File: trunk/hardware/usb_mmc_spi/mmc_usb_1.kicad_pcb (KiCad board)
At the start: 2 copper layers, 47.6 x 27.3 mm, 25 parts, among them J301 MINI-USB-5P-3400020P1, K301 CONN_3, P301 CONN_5X2, P302 MICRO-SDCARD-CONNECTOR-330006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, P303 CONN_10X2, P304 CONN_10X2, P305 CONN_1, P306 CONN_1, U301 FT232RL

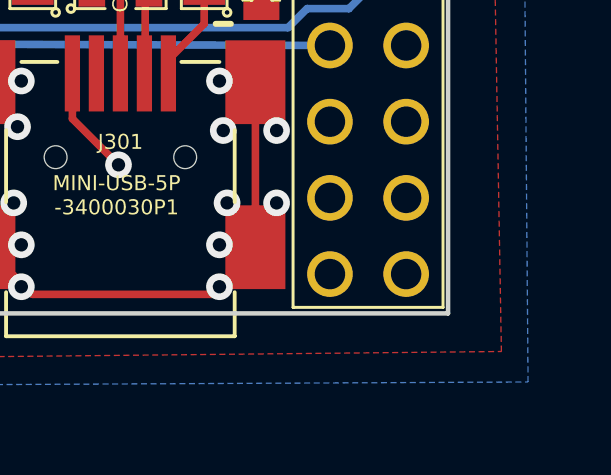
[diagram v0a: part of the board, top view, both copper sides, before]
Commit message: bugfix
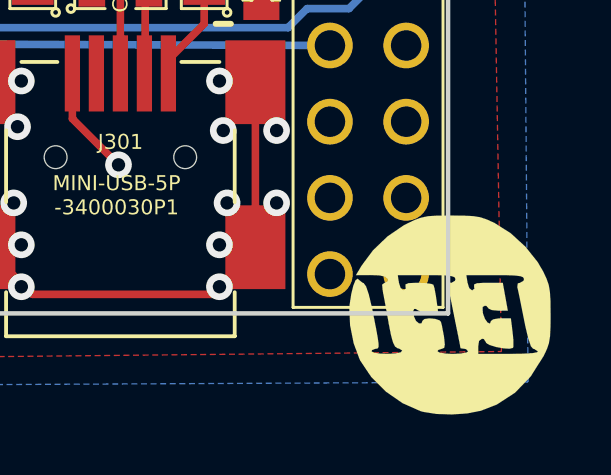
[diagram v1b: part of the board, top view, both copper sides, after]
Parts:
- added G301: LOGO, LOGO_F, F.Cu at (224.1, 179.2)
- renumbered G301 to G3
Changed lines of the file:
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@@
     (links 76)
     (no_connects 0)
-    (area 120.549999 93.244999 233.0704 190.600001)
+    (area 176.327999 151.689999 224.103001 179.145001)
     (thickness 1.6)
     (drawings 62)
     (tracks 536)
     (zones 0)
-    (modules 25)
+    (modules 26)
     (nets 24)
   )
@@
       (layers F.Cu F.Paste F.Mask)
     )
-    (pad G301 smd rect (at -6.893 8.032 270) (size 1.524 1.016)
+    (pad G3 smd rect (at -6.893 8.032 270) (size 1.524 1.016)
       (layers F.Cu F.Paste F.Mask)
       (net 13 GND)
@@
   (module LOGO_F (layer B.Cu)
     (at 201.549 165.608)
-    (fp_text reference G301 (at 0 -4.14782) (layer B.SilkS) hide
+    (fp_text reference G3 (at 0 -4.14782) (layer B.SilkS) hide
       (effects (font (size 1.524 1.524) (thickness 0.3048)) (justify mirror))
     )
@@
     )
   )
+  (module LOGO_F (layer F.Cu)
+    (at 224.103001 179.150001)
+    (fp_text reference G301 (at 0 4.14782) (layer F.SilkS) hide
+      (effects (font (size 1.524 1.524) (thickness 0.3048)))
+    )
+    (fp_text value LOGO (at 0 -4.14782) (layer F.SilkS) hide
+      (effects (font (size 1.524 1.524) (thickness 0.3048)))
+    )
+    (fp_poly (pts (xy 3.34518 -0.04318) (xy 3.3401 0.381) (xy 3.32486 0.68326) (xy 3.28676 0.90932)
+      (xy 3.22326 1.1049) (xy 3.12166 1.3208) (xy 3.10896 1.3462) (xy 2.921 1.64084)
+      (xy 2.921 1.18618) (xy 2.79654 1.1049) (xy 2.75844 1.09982) (xy 2.68732 1.016)
+      (xy 2.60096 0.76708) (xy 2.5019 0.35052) (xy 2.46126 0.14732) (xy 2.38252 -0.24638)
+      (xy 2.31394 -0.58928) (xy 2.2606 -0.84074) (xy 2.23266 -0.9525) (xy 2.2479 -1.07696)
+      (xy 2.32156 -1.09982) (xy 2.4384 -1.16586) (xy 2.45618 -1.22682) (xy 2.42824 -1.28524)
+      (xy 2.33172 -1.3208) (xy 2.13868 -1.34366) (xy 1.82372 -1.35382) (xy 1.49606 -1.35382)
+      (xy 0.53594 -1.35382) (xy 0.57404 -1.09982) (xy 0.63246 -0.92202) (xy 0.7239 -0.84836)
+      (xy 0.72644 -0.84582) (xy 0.80264 -0.90678) (xy 0.79248 -0.97536) (xy 0.79248 -1.04648)
+      (xy 0.889 -1.08458) (xy 1.10744 -1.09982) (xy 1.24714 -1.09982) (xy 1.75006 -1.09982)
+      (xy 1.83388 -0.635) (xy 1.9177 -0.17018) (xy 1.59258 -0.17018) (xy 1.38684 -0.1905)
+      (xy 1.27508 -0.23876) (xy 1.27 -0.254) (xy 1.20142 -0.3302) (xy 1.15316 -0.33782)
+      (xy 1.0795 -0.2921) (xy 1.08204 -0.127) (xy 1.0922 -0.07112) (xy 1.1557 0.1016)
+      (xy 1.24206 0.22352) (xy 1.3208 0.25908) (xy 1.35382 0.1778) (xy 1.35382 0.17526)
+      (xy 1.43002 0.11684) (xy 1.61544 0.08636) (xy 1.68656 0.08382) (xy 2.0193 0.08382)
+      (xy 2.07772 0.55372) (xy 2.10312 0.81788) (xy 2.10312 1.01092) (xy 2.09042 1.06934)
+      (xy 1.9685 1.09982) (xy 1.76022 1.08458) (xy 1.52146 1.03886) (xy 1.31318 0.97536)
+      (xy 1.1938 0.90424) (xy 1.18618 0.88138) (xy 1.1176 0.7747) (xy 1.05918 0.762)
+      (xy 0.95758 0.8382) (xy 0.93218 1.016) (xy 0.93218 1.27) (xy 1.95072 1.27)
+      (xy 2.42062 1.26238) (xy 2.74066 1.2446) (xy 2.90322 1.21158) (xy 2.921 1.18618)
+      (xy 2.921 1.64084) (xy 2.67716 2.02692) (xy 2.15646 2.5654) (xy 1.5494 2.9591)
+      (xy 1.02108 3.16484) (xy 0.59182 3.24866) (xy 0.59182 1.18618) (xy 0.52324 1.10998)
+      (xy 0.46482 1.09982) (xy 0.35306 1.08458) (xy 0.33782 1.06934) (xy 0.32258 0.98044)
+      (xy 0.2794 0.75692) (xy 0.21336 0.4318) (xy 0.13462 0.04064) (xy 0.127 0)
+      (xy 0.03556 -0.44958) (xy -0.02794 -0.75692) (xy -0.06096 -0.94996) (xy -0.06858 -1.0541)
+      (xy -0.05334 -1.09728) (xy -0.01524 -1.1049) (xy 0.04318 -1.09982) (xy 0.15494 -1.1684)
+      (xy 0.17018 -1.22682) (xy 0.14224 -1.28524) (xy 0.04572 -1.3208) (xy -0.14732 -1.34366)
+      (xy -0.46228 -1.35382) (xy -0.78994 -1.35382) (xy -1.75006 -1.35382) (xy -1.71196 -1.09982)
+      (xy -1.65354 -0.92202) (xy -1.5621 -0.84836) (xy -1.55956 -0.84582) (xy -1.48336 -0.90678)
+      (xy -1.49352 -0.97282) (xy -1.49098 -1.04902) (xy -1.39446 -1.08712) (xy -1.1684 -1.09982)
+      (xy -1.07188 -1.09982) (xy -0.80772 -1.08966) (xy -0.61976 -1.05918) (xy -0.56134 -1.03378)
+      (xy -0.52578 -0.9144) (xy -0.48514 -0.69088) (xy -0.45974 -0.52578) (xy -0.40132 -0.08382)
+      (xy -0.69342 -0.08382) (xy -0.91948 -0.11176) (xy -1.07696 -0.18034) (xy -1.08204 -0.18542)
+      (xy -1.1938 -0.254) (xy -1.2319 -0.17018) (xy -1.21158 0.02032) (xy -1.143 0.17018)
+      (xy -1.04394 0.254) (xy -0.95758 0.24892) (xy -0.93218 0.17018) (xy -0.86106 0.10668)
+      (xy -0.69596 0.08382) (xy -0.50546 0.1016) (xy -0.35306 0.15494) (xy -0.31242 0.20066)
+      (xy -0.27432 0.35052) (xy -0.2286 0.59436) (xy -0.20828 0.70866) (xy -0.18288 0.94996)
+      (xy -0.20066 1.0668) (xy -0.27686 1.09982) (xy -0.28702 1.09982) (xy -0.4064 1.143)
+      (xy -0.42418 1.18618) (xy -0.34544 1.22936) (xy -0.14478 1.25984) (xy 0.08382 1.27)
+      (xy 0.3556 1.2573) (xy 0.53848 1.22428) (xy 0.59182 1.18618) (xy 0.59182 3.24866)
+      (xy 0.5715 3.25374) (xy 0.0508 3.2893) (xy -0.4699 3.27152) (xy -0.91694 3.2004)
+      (xy -0.99314 3.17754) (xy -1.59004 2.91338) (xy -2.15392 2.52222) (xy -2.63652 2.03708)
+      (xy -2.99974 1.49606) (xy -3.03022 1.43256) (xy -3.22326 0.90932) (xy -3.3401 0.32258)
+      (xy -3.3655 -0.2413) (xy -3.3528 -0.39624) (xy -3.29946 -0.7366) (xy -3.23088 -1.01092)
+      (xy -3.15722 -1.18872) (xy -3.0861 -1.23698) (xy -3.06578 -1.21666) (xy -2.93624 -1.10998)
+      (xy -2.88544 -1.08712) (xy -2.80924 -0.98298) (xy -2.7178 -0.71374) (xy -2.6162 -0.2921)
+      (xy -2.57302 -0.08128) (xy -2.48158 0.38354) (xy -2.42316 0.70612) (xy -2.39268 0.9144)
+      (xy -2.39014 1.03124) (xy -2.41554 1.08458) (xy -2.4638 1.09982) (xy -2.49682 1.09982)
+      (xy -2.61112 1.14554) (xy -2.62382 1.18618) (xy -2.54762 1.22936) (xy -2.34696 1.25984)
+      (xy -2.11582 1.27) (xy -1.8288 1.25476) (xy -1.651 1.21412) (xy -1.60274 1.15824)
+      (xy -1.7018 1.09728) (xy -1.76276 1.0795) (xy -1.8415 1.02362) (xy -1.91008 0.88646)
+      (xy -1.97866 0.63754) (xy -2.05486 0.25146) (xy -2.06248 0.2032) (xy -2.13106 -0.18288)
+      (xy -2.19456 -0.52578) (xy -2.24282 -0.78232) (xy -2.25806 -0.86868) (xy -2.27076 -1.0414)
+      (xy -2.19202 -1.09982) (xy -2.1717 -1.10236) (xy -2.07772 -1.15316) (xy -2.08534 -1.22936)
+      (xy -2.1717 -1.30556) (xy -2.36728 -1.3462) (xy -2.6416 -1.35636) (xy -3.14706 -1.35382)
+      (xy -2.95656 -1.67132) (xy -2.5781 -2.18186) (xy -2.09296 -2.64668) (xy -1.55702 -3.01244)
+      (xy -1.44018 -3.0734) (xy -1.18618 -3.19532) (xy -0.97536 -3.27152) (xy -0.75692 -3.31724)
+      (xy -0.48514 -3.33756) (xy -0.10668 -3.34264) (xy 0.04064 -3.34264) (xy 0.46482 -3.33756)
+      (xy 0.76962 -3.32232) (xy 1.00076 -3.28422) (xy 1.2065 -3.21564) (xy 1.43764 -3.1115)
+      (xy 1.47574 -3.09372) (xy 2.00914 -2.7559) (xy 2.50444 -2.30378) (xy 2.91592 -1.78816)
+      (xy 3.10134 -1.46812) (xy 3.21056 -1.2319) (xy 3.28168 -1.02616) (xy 3.31978 -0.8001)
+      (xy 3.3401 -0.50546) (xy 3.34264 -0.09398) (xy 3.34518 -0.04318) (xy 3.34518 -0.04318)) (layer F.SilkS) (width 0.00254))
+  )
   (gr_text 6 (at 215.519 158.623) (layer B.SilkS)

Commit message: kinda fixing the whole G* situation
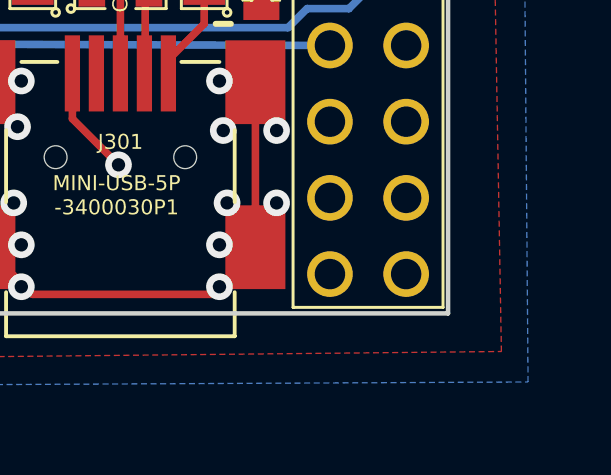
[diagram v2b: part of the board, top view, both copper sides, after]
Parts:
- removed G301: LOGO, LOGO_F
- renumbered G3 to G305
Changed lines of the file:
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@@
     (links 76)
     (no_connects 0)
-    (area 176.327999 151.689999 224.103001 179.145001)
+    (area 120.549999 93.244999 233.0704 190.600001)
     (thickness 1.6)
     (drawings 62)
     (tracks 536)
     (zones 0)
-    (modules 26)
+    (modules 25)
     (nets 24)
   )
@@
       (layers F.Cu F.Paste F.Mask)
     )
-    (pad G3 smd rect (at -6.893 8.032 270) (size 1.524 1.016)
-      (layers F.Cu F.Paste F.Mask)
-      (net 13 GND)
-    )
-    (pad G2 smd rect (at 2.88 7.686 270) (size 2.032 1.524)
-      (layers F.Cu F.Paste F.Mask)
-      (net 13 GND)
-    )
-    (pad G3 smd rect (at 2.88 -7.714 270) (size 2.032 1.524)
-      (layers F.Cu F.Paste F.Mask)
-      (net 13 GND)
-    )
-    (pad G4 smd rect (at -7.101 -6.895 270) (size 1.524 1.524)
+    (pad G301 smd rect (at -6.893 8.032 270) (size 1.524 1.016)
+      (layers F.Cu F.Paste F.Mask)
+      (net 13 GND)
+    )
+    (pad G302 smd rect (at 2.88 7.686 270) (size 2.032 1.524)
+      (layers F.Cu F.Paste F.Mask)
+      (net 13 GND)
+    )
+    (pad G303 smd rect (at 2.88 -7.714 270) (size 2.032 1.524)
+      (layers F.Cu F.Paste F.Mask)
+      (net 13 GND)
+    )
+    (pad G304 smd rect (at -7.101 -6.895 270) (size 1.524 1.524)
       (layers F.Cu F.Paste F.Mask)
       (net 13 GND)
@@
   (module LOGO_F (layer B.Cu)
     (at 201.549 165.608)
-    (fp_text reference G3 (at 0 -4.14782) (layer B.SilkS) hide
+    (fp_text reference G305 (at 0 -4.14782) (layer B.SilkS) hide
       (effects (font (size 1.524 1.524) (thickness 0.3048)) (justify mirror))
     )
@@
     )
   )
-  (module LOGO_F (layer F.Cu)
-    (at 224.103001 179.150001)
-    (fp_text reference G301 (at 0 4.14782) (layer F.SilkS) hide
-      (effects (font (size 1.524 1.524) (thickness 0.3048)))
-    )
-    (fp_text value LOGO (at 0 -4.14782) (layer F.SilkS) hide
-      (effects (font (size 1.524 1.524) (thickness 0.3048)))
-    )
-    (fp_poly (pts (xy 3.34518 -0.04318) (xy 3.3401 0.381) (xy 3.32486 0.68326) (xy 3.28676 0.90932)
-      (xy 3.22326 1.1049) (xy 3.12166 1.3208) (xy 3.10896 1.3462) (xy 2.921 1.64084)
-      (xy 2.921 1.18618) (xy 2.79654 1.1049) (xy 2.75844 1.09982) (xy 2.68732 1.016)
-      (xy 2.60096 0.76708) (xy 2.5019 0.35052) (xy 2.46126 0.14732) (xy 2.38252 -0.24638)
-      (xy 2.31394 -0.58928) (xy 2.2606 -0.84074) (xy 2.23266 -0.9525) (xy 2.2479 -1.07696)
-      (xy 2.32156 -1.09982) (xy 2.4384 -1.16586) (xy 2.45618 -1.22682) (xy 2.42824 -1.28524)
-      (xy 2.33172 -1.3208) (xy 2.13868 -1.34366) (xy 1.82372 -1.35382) (xy 1.49606 -1.35382)
-      (xy 0.53594 -1.35382) (xy 0.57404 -1.09982) (xy 0.63246 -0.92202) (xy 0.7239 -0.84836)
-      (xy 0.72644 -0.84582) (xy 0.80264 -0.90678) (xy 0.79248 -0.97536) (xy 0.79248 -1.04648)
-      (xy 0.889 -1.08458) (xy 1.10744 -1.09982) (xy 1.24714 -1.09982) (xy 1.75006 -1.09982)
-      (xy 1.83388 -0.635) (xy 1.9177 -0.17018) (xy 1.59258 -0.17018) (xy 1.38684 -0.1905)
-      (xy 1.27508 -0.23876) (xy 1.27 -0.254) (xy 1.20142 -0.3302) (xy 1.15316 -0.33782)
-      (xy 1.0795 -0.2921) (xy 1.08204 -0.127) (xy 1.0922 -0.07112) (xy 1.1557 0.1016)
-      (xy 1.24206 0.22352) (xy 1.3208 0.25908) (xy 1.35382 0.1778) (xy 1.35382 0.17526)
-      (xy 1.43002 0.11684) (xy 1.61544 0.08636) (xy 1.68656 0.08382) (xy 2.0193 0.08382)
-      (xy 2.07772 0.55372) (xy 2.10312 0.81788) (xy 2.10312 1.01092) (xy 2.09042 1.06934)
-      (xy 1.9685 1.09982) (xy 1.76022 1.08458) (xy 1.52146 1.03886) (xy 1.31318 0.97536)
-      (xy 1.1938 0.90424) (xy 1.18618 0.88138) (xy 1.1176 0.7747) (xy 1.05918 0.762)
-      (xy 0.95758 0.8382) (xy 0.93218 1.016) (xy 0.93218 1.27) (xy 1.95072 1.27)
-      (xy 2.42062 1.26238) (xy 2.74066 1.2446) (xy 2.90322 1.21158) (xy 2.921 1.18618)
-      (xy 2.921 1.64084) (xy 2.67716 2.02692) (xy 2.15646 2.5654) (xy 1.5494 2.9591)
-      (xy 1.02108 3.16484) (xy 0.59182 3.24866) (xy 0.59182 1.18618) (xy 0.52324 1.10998)
-      (xy 0.46482 1.09982) (xy 0.35306 1.08458) (xy 0.33782 1.06934) (xy 0.32258 0.98044)
-      (xy 0.2794 0.75692) (xy 0.21336 0.4318) (xy 0.13462 0.04064) (xy 0.127 0)
-      (xy 0.03556 -0.44958) (xy -0.02794 -0.75692) (xy -0.06096 -0.94996) (xy -0.06858 -1.0541)
-      (xy -0.05334 -1.09728) (xy -0.01524 -1.1049) (xy 0.04318 -1.09982) (xy 0.15494 -1.1684)
-      (xy 0.17018 -1.22682) (xy 0.14224 -1.28524) (xy 0.04572 -1.3208) (xy -0.14732 -1.34366)
-      (xy -0.46228 -1.35382) (xy -0.78994 -1.35382) (xy -1.75006 -1.35382) (xy -1.71196 -1.09982)
-      (xy -1.65354 -0.92202) (xy -1.5621 -0.84836) (xy -1.55956 -0.84582) (xy -1.48336 -0.90678)
-      (xy -1.49352 -0.97282) (xy -1.49098 -1.04902) (xy -1.39446 -1.08712) (xy -1.1684 -1.09982)
-      (xy -1.07188 -1.09982) (xy -0.80772 -1.08966) (xy -0.61976 -1.05918) (xy -0.56134 -1.03378)
-      (xy -0.52578 -0.9144) (xy -0.48514 -0.69088) (xy -0.45974 -0.52578) (xy -0.40132 -0.08382)
-      (xy -0.69342 -0.08382) (xy -0.91948 -0.11176) (xy -1.07696 -0.18034) (xy -1.08204 -0.18542)
-      (xy -1.1938 -0.254) (xy -1.2319 -0.17018) (xy -1.21158 0.02032) (xy -1.143 0.17018)
-      (xy -1.04394 0.254) (xy -0.95758 0.24892) (xy -0.93218 0.17018) (xy -0.86106 0.10668)
-      (xy -0.69596 0.08382) (xy -0.50546 0.1016) (xy -0.35306 0.15494) (xy -0.31242 0.20066)
-      (xy -0.27432 0.35052) (xy -0.2286 0.59436) (xy -0.20828 0.70866) (xy -0.18288 0.94996)
-      (xy -0.20066 1.0668) (xy -0.27686 1.09982) (xy -0.28702 1.09982) (xy -0.4064 1.143)
-      (xy -0.42418 1.18618) (xy -0.34544 1.22936) (xy -0.14478 1.25984) (xy 0.08382 1.27)
-      (xy 0.3556 1.2573) (xy 0.53848 1.22428) (xy 0.59182 1.18618) (xy 0.59182 3.24866)
-      (xy 0.5715 3.25374) (xy 0.0508 3.2893) (xy -0.4699 3.27152) (xy -0.91694 3.2004)
-      (xy -0.99314 3.17754) (xy -1.59004 2.91338) (xy -2.15392 2.52222) (xy -2.63652 2.03708)
-      (xy -2.99974 1.49606) (xy -3.03022 1.43256) (xy -3.22326 0.90932) (xy -3.3401 0.32258)
-      (xy -3.3655 -0.2413) (xy -3.3528 -0.39624) (xy -3.29946 -0.7366) (xy -3.23088 -1.01092)
-      (xy -3.15722 -1.18872) (xy -3.0861 -1.23698) (xy -3.06578 -1.21666) (xy -2.93624 -1.10998)
-      (xy -2.88544 -1.08712) (xy -2.80924 -0.98298) (xy -2.7178 -0.71374) (xy -2.6162 -0.2921)
-      (xy -2.57302 -0.08128) (xy -2.48158 0.38354) (xy -2.42316 0.70612) (xy -2.39268 0.9144)
-      (xy -2.39014 1.03124) (xy -2.41554 1.08458) (xy -2.4638 1.09982) (xy -2.49682 1.09982)
-      (xy -2.61112 1.14554) (xy -2.62382 1.18618) (xy -2.54762 1.22936) (xy -2.34696 1.25984)
-      (xy -2.11582 1.27) (xy -1.8288 1.25476) (xy -1.651 1.21412) (xy -1.60274 1.15824)
-      (xy -1.7018 1.09728) (xy -1.76276 1.0795) (xy -1.8415 1.02362) (xy -1.91008 0.88646)
-      (xy -1.97866 0.63754) (xy -2.05486 0.25146) (xy -2.06248 0.2032) (xy -2.13106 -0.18288)
-      (xy -2.19456 -0.52578) (xy -2.24282 -0.78232) (xy -2.25806 -0.86868) (xy -2.27076 -1.0414)
-      (xy -2.19202 -1.09982) (xy -2.1717 -1.10236) (xy -2.07772 -1.15316) (xy -2.08534 -1.22936)
-      (xy -2.1717 -1.30556) (xy -2.36728 -1.3462) (xy -2.6416 -1.35636) (xy -3.14706 -1.35382)
-      (xy -2.95656 -1.67132) (xy -2.5781 -2.18186) (xy -2.09296 -2.64668) (xy -1.55702 -3.01244)
-      (xy -1.44018 -3.0734) (xy -1.18618 -3.19532) (xy -0.97536 -3.27152) (xy -0.75692 -3.31724)
-      (xy -0.48514 -3.33756) (xy -0.10668 -3.34264) (xy 0.04064 -3.34264) (xy 0.46482 -3.33756)
-      (xy 0.76962 -3.32232) (xy 1.00076 -3.28422) (xy 1.2065 -3.21564) (xy 1.43764 -3.1115)
-      (xy 1.47574 -3.09372) (xy 2.00914 -2.7559) (xy 2.50444 -2.30378) (xy 2.91592 -1.78816)
-      (xy 3.10134 -1.46812) (xy 3.21056 -1.2319) (xy 3.28168 -1.02616) (xy 3.31978 -0.8001)
-      (xy 3.3401 -0.50546) (xy 3.34264 -0.09398) (xy 3.34518 -0.04318) (xy 3.34518 -0.04318)) (layer F.SilkS) (width 0.00254))
-  )
   (gr_text 6 (at 215.519 158.623) (layer B.SilkS)
